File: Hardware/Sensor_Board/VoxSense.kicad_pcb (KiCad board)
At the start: 4 copper layers, 85 x 15.7 mm, 94 parts, among them J301 TC2030-NL, J302 PicoBlade, J501 RJ45_Input, J502 RJ45_Output, SW301 Reset, SW501 Slide Switch, U101 TPS25942ARVCR, U201 TPS7A20L_1V2, U202 TPS7A20L_2V2, U203 TPS7A20L_3V3, U204 TLV840, U301 ICE40UL1K-CM36AI, U302 TPD4E02B04, U305 N25Q032A, U401 BNO086, U501 TPD4E02B04, U502 TPD4E02B04, U503 TPD4E02B04, U504 TPD4E02B04, U505 CBTU02044, Y301 ASCO, Y401 32.768 kHz

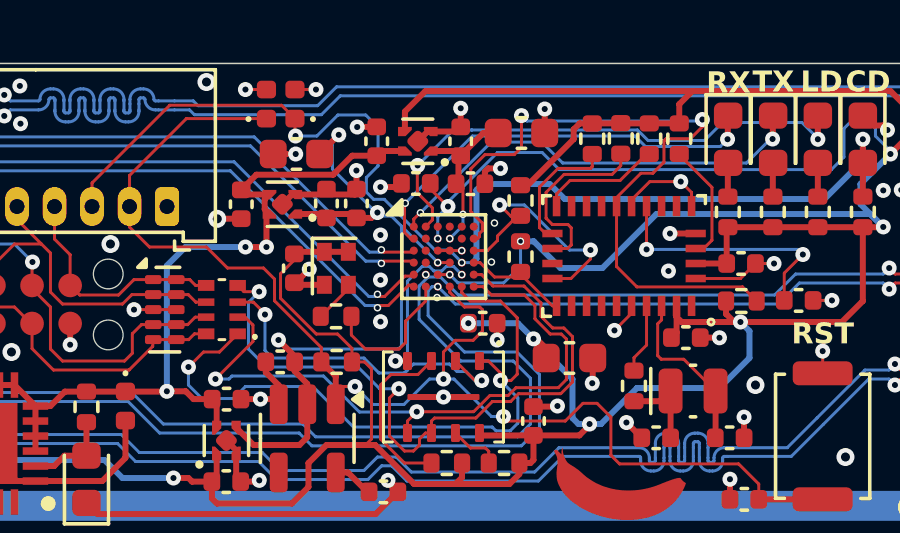
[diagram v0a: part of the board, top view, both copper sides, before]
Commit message: Commited the final manufacturing files, as well as updated the documentation
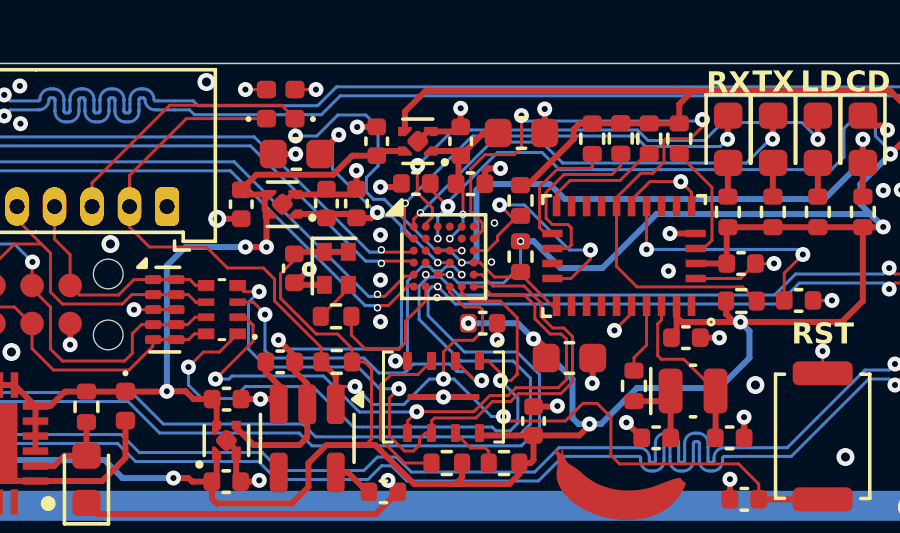
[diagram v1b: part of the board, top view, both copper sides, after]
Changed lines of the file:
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@@
 		)
 		(fp_line
-			(start -2.25 -2.25)
-			(end -2.25 2.25)
+			(start -1.7 -1.7)
+			(end -1.7 1.7)
 			(stroke
 				(width 0.05)
@@
 		)
 		(fp_line
-			(start -2.25 2.25)
-			(end 2.25 2.25)
+			(start -1.7 1.7)
+			(end 1.7 1.7)
 			(stroke
 				(width 0.05)
@@
 		)
 		(fp_line
-			(start 2.25 -2.25)
-			(end -2.25 -2.25)
+			(start 1.7 -1.7)
+			(end -1.7 -1.7)
 			(stroke
 				(width 0.05)
@@
 		)
 		(fp_line
-			(start 2.25 2.25)
-			(end 2.25 -2.25)
+			(start 1.7 1.7)
+			(end 1.7 -1.7)
 			(stroke
 				(width 0.05)
@@
 	)
 	(segment
-		(start 113.332327 69.796022)
-		(end 113.332327 70.197673)
+		(start 113.332327 70.1)
+		(end 113.11 70.322327)
 		(width 0.1)
 		(layer "F.Cu")
@@
 	)
 	(segment
-		(start 112.83 69.293695)
-		(end 113.332327 69.796022)
+		(start 112.84 68.38)
+		(end 112.83 68.39)
 		(width 0.1)
 		(layer "F.Cu")
@@
 	)
 	(segment
-		(start 112.84 68.38)
-		(end 112.83 68.39)
+		(start 113.332327 69.796022)
+		(end 113.332327 70.1)
 		(width 0.1)
 		(layer "F.Cu")
@@
 	)
 	(segment
+		(start 126.18 66.72)
+		(end 126.18 67.5075)
+		(width 0.2)
+		(layer "F.Cu")
+		(net 15)
+	)
+	(segment
 		(start 112.83 68.39)
 		(end 112.83 69.293695)
@@
 	)
 	(segment
-		(start 113.332327 70.197673)
+		(start 113.11 70.322327)
 		(end 113.11 70.42)
 		(width 0.1)
@@
 	)
 	(segment
-		(start 126.18 66.72)
-		(end 126.18 67.5075)
-		(width 0.2)
+		(start 112.83 69.293695)
+		(end 113.332327 69.796022)
+		(width 0.1)
 		(layer "F.Cu")
 		(net 15)
@@
 	)
 	(segment
-		(start 126.18 67.48)
-		(end 126.18 67.5075)
+		(start 125.65 66.95)
+		(end 126.18 67.48)
 		(width 0.1)
 		(layer "B.Cu")
@@
 	)
 	(segment
-		(start 114.02 67.2)
-		(end 114.642138 67.2)
+		(start 114.021 67.199)
+		(end 112.84 68.38)
 		(width 0.1)
 		(layer "B.Cu")
@@
 	)
 	(segment
-		(start 114.642138 67.2)
-		(end 114.643138 67.199)
+		(start 122.401 67.549)
+		(end 123 66.95)
 		(width 0.1)
 		(layer "B.Cu")
@@
 	)
 	(segment
-		(start 120.518256 67.549)
-		(end 122.401 67.549)
-		(width 0.1)
-		(layer "B.Cu")
-		(net 15)
-	)
-	(segment
-		(start 125.65 66.95)
-		(end 126.18 67.48)
+		(start 126.18 67.48)
+		(end 126.18 67.5075)
 		(width 0.1)
 		(layer "B.Cu")
@@
 	)
 	(segment
-		(start 122.401 67.549)
-		(end 123 66.95)
+		(start 120.168256 67.199)
+		(end 120.518256 67.549)
 		(width 0.1)
 		(layer "B.Cu")
@@
 	)
 	(segment
-		(start 120.168256 67.199)
-		(end 120.518256 67.549)
+		(start 120.518256 67.549)
+		(end 122.401 67.549)
 		(width 0.1)
 		(layer "B.Cu")
@@
 	)
 	(segment
-		(start 112.84 68.38)
-		(end 114.02 67.2)
+		(start 114.643138 67.199)
+		(end 114.021 67.199)
 		(width 0.1)
 		(layer "B.Cu")
@@
 	)
 	(segment
+		(start 114.996 70.554)
+		(end 114.73 70.82)
+		(width 0.1)
+		(layer "F.Cu")
+		(net 38)
+	)
+	(segment
 		(start 121.93 67.49)
 		(end 121.12 67.49)
@@
 	)
 	(segment
-		(start 116.3 66.72)
-		(end 116.3 67.78)
+		(start 115.0829 68.02)
+		(end 114.61 68.4929)
 		(width 0.1)
 		(layer "F.Cu")
@@
 	)
 	(segment
-		(start 121.12 67.49)
-		(end 121.05 67.56)
+		(start 116.3 67.78)
+		(end 116.06 68.02)
 		(width 0.1)
 		(layer "F.Cu")
@@
 	)
 	(segment
-		(start 119.47 71.75)
-		(end 120.15 72.43)
+		(start 114.61 69.915534)
+		(end 114.996 70.301534)
 		(width 0.1)
 		(layer "F.Cu")
@@
 	)
 	(segment
-		(start 114.61 68.4929)
-		(end 114.61 69.915534)
+		(start 121.12 67.49)
+		(end 121.05 67.56)
+		(width 0.1)
+		(layer "F.Cu")
+		(net 38)
+	)
+	(segment
+		(start 119.47 71.75)
+		(end 120.15 72.43)
 		(width 0.1)
 		(layer "F.Cu")
@@
 	)
 	(segment
-		(start 119.47 69.452128)
-		(end 119.47 69.7375)
+		(start 114.73 70.82)
+		(end 114.71 70.82)
 		(width 0.1)
 		(layer "F.Cu")
@@
 	)
 	(segment
-		(start 116.3 67.78)
-		(end 116.06 68.02)
+		(start 114.61 68.4929)
+		(end 114.61 69.915534)
 		(width 0.1)
 		(layer "F.Cu")
@@
 	)
 	(segment
-		(start 115.0829 68.02)
-		(end 114.61 68.4929)
+		(start 119.47 69.452128)
+		(end 119.47 69.7375)
 		(width 0.1)
 		(layer "F.Cu")
@@
 	)
 	(segment
-		(start 114.9 70.75)
-		(end 114.83 70.82)
+		(start 116.3 66.72)
+		(end 116.3 67.78)
 		(width 0.1)
 		(layer "F.Cu")
@@
 	)
 	(segment
-		(start 114.61 69.915534)
-		(end 114.996 70.301534)
+		(start 116.06 68.02)
+		(end 115.0829 68.02)
 		(width 0.1)
 		(layer "F.Cu")
@@
 	)
 	(segment
-		(start 114.996 70.301534)
-		(end 114.996 70.554)
-		(width 0.1)
-		(layer "F.Cu")
-		(net 38)
-	)
-	(segment
-		(start 114.83 70.82)
-		(end 114.71 70.82)
-		(width 0.1)
-		(layer "F.Cu")
-		(net 38)
-	)
-	(segment
 		(start 124.14 72.9)
 		(end 123.67 72.43)
@@
 	)
 	(segment
-		(start 114.9 70.65)
-		(end 114.9 70.75)
-		(width 0.1)
-		(layer "F.Cu")
-		(net 38)
-	)
-	(segment
-		(start 114.996 70.554)
-		(end 114.9 70.65)
-		(width 0.1)
-		(layer "F.Cu")
-		(net 38)
-	)
-	(segment
-		(start 116.06 68.02)
-		(end 115.0829 68.02)
+		(start 114.996 70.301534)
+		(end 114.996 70.554)
 		(width 0.1)
 		(layer "F.Cu")
@@
 		(width 0.1)
 		(layer "F.Cu")
-		(net 52)
-	)
-	(segment
-		(start 112.956073 73.051964)
-		(end 112.954018 73.054018)
-		(width 0.1)
-		(layer "F.Cu")
